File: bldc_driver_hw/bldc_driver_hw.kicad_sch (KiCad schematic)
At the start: 28 parts, among them J1 Conn_01x02, J10 MR60_F, J2 USB_C_Receptacle_USB2.0_16P, J3 JTAG_CONN, J4 USB_C_Receptacle_USB2.0_16P, J5 Conn_01x03_Pin, J6 Conn_01x03_Pin, J7 Conn_01x03, J9 Conn_01x02, U2 USBLC6-2SC6, U7 USBLC6-2SC6

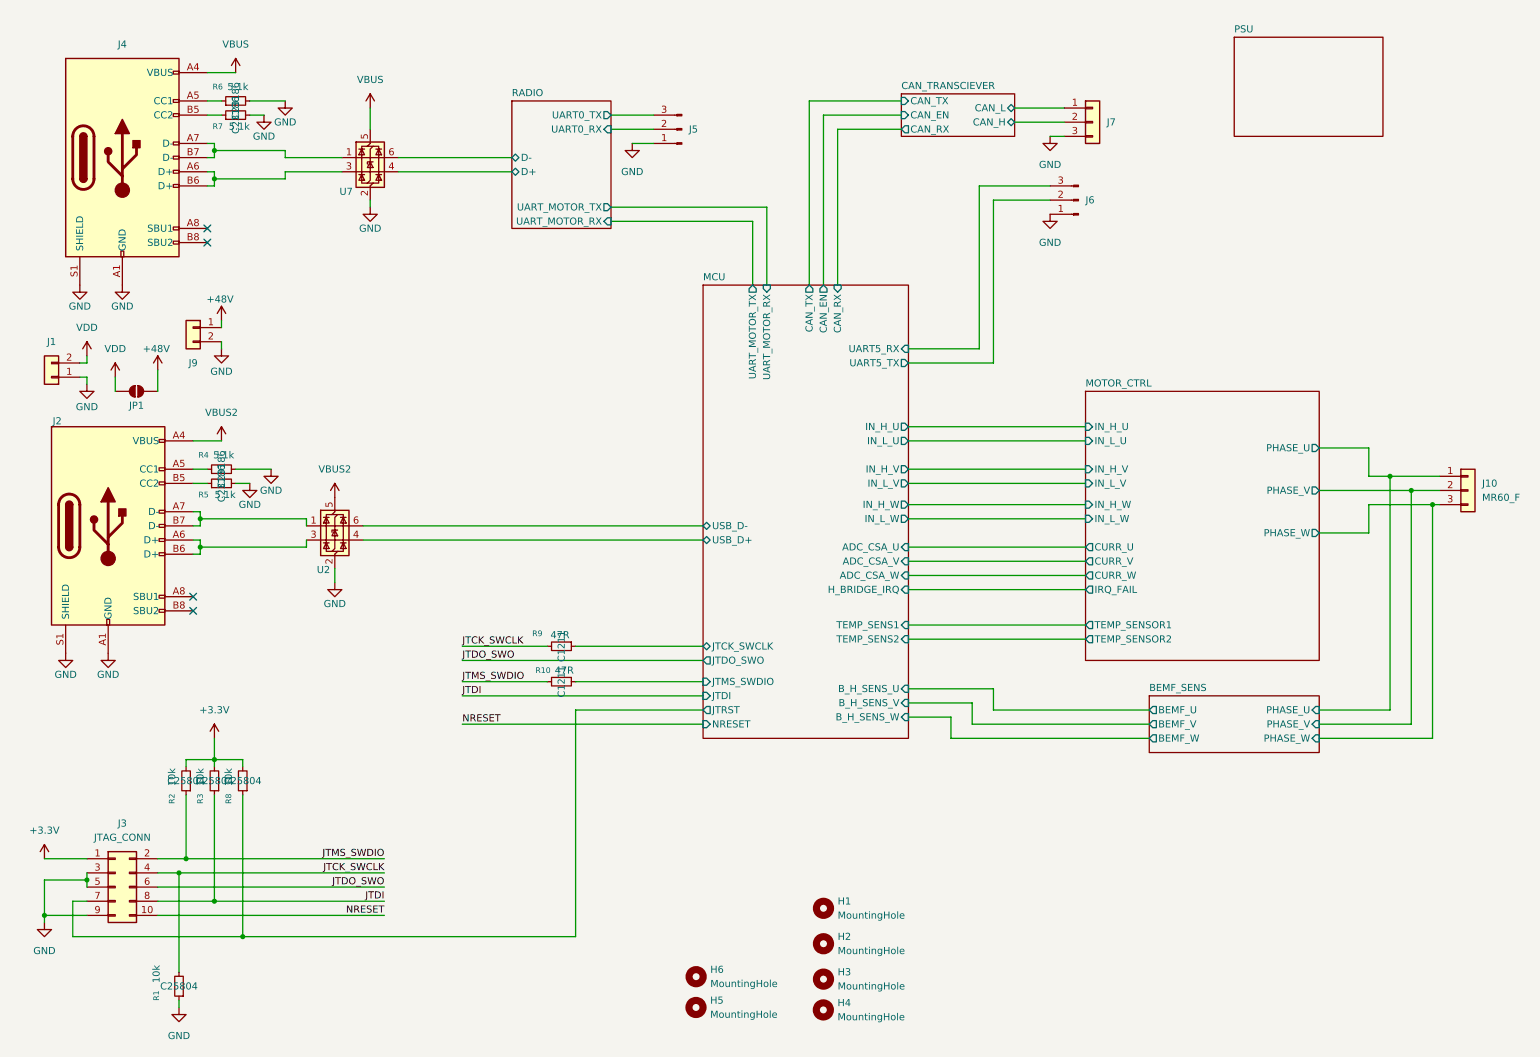
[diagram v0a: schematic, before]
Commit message: finished_board
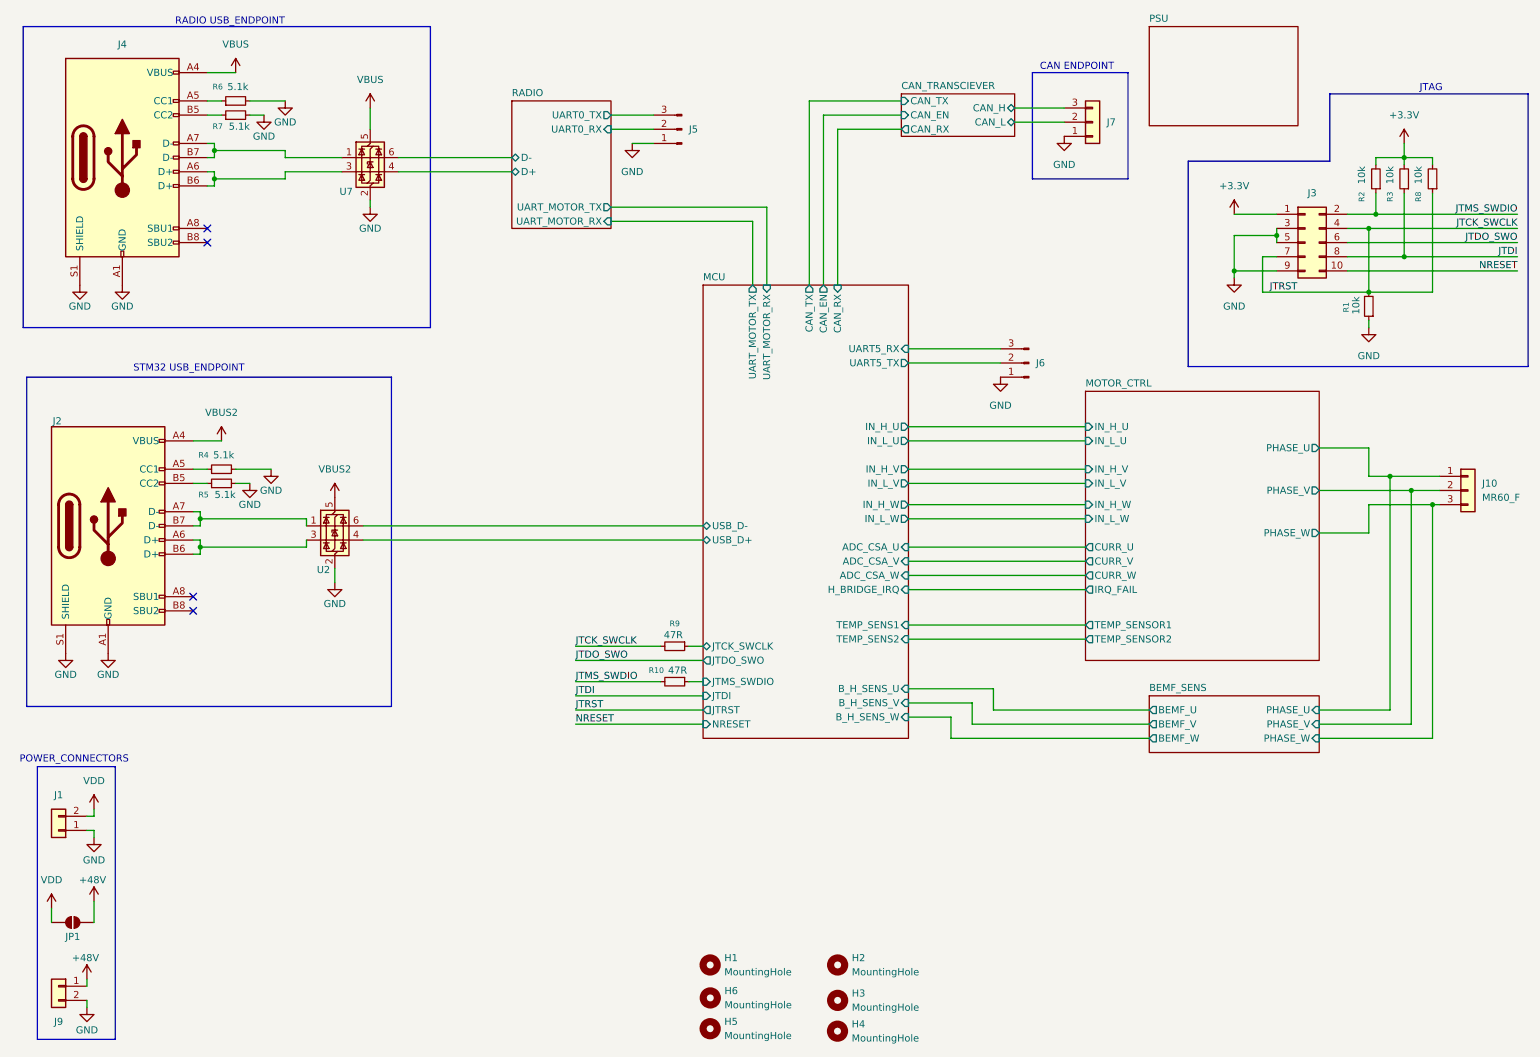
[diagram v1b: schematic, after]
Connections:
- net MCU/JTRST is gone; now on net JTCK_SWCLK: J3.7 (Pin_7), R8.1
- net CAN_TRANSCIEVER/CAN_H: now also J7.3 (Pin_3); no longer J7.2 (Pin_2)
- net CAN_TRANSCIEVER/CAN_L: now also J7.2 (Pin_2); no longer J7.1 (Pin_1)
- net GND: now also J7.1 (Pin_1); no longer J7.3 (Pin_3)
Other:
- note added: "CAN ENDPOINT"
- note added: "JTAG"
- note added: "POWER_CONNECTORS"
- note added: "RADIO USB_ENDPOINT"
- note added: "STM32 USB_ENDPOINT"
- moved on the sheet: H1, H2, H3, H4, H5, H6, J1, J3, J6, J9, JP1, R1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

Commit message: finished
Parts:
- J1, J10, J2, J3, J4, J5, J6, J7, J9, U2, U7: now left out of the parts list
- R10, R9: LCSC C1211 -> C23182
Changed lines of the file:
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@@
 		(unit 1)
 		(exclude_from_sim no)
-		(in_bom yes)
+		(in_bom no)
 		(on_board yes)
 		(dnp no)
@@
 			)
 		)
-		(property "LCSC" "C1211"
+		(property "LCSC" "C23182"
 			(at 130.81 132.08 0)
 			(effects
@@
 		(unit 1)
 		(exclude_from_sim no)
-		(in_bom yes)
+		(in_bom no)
 		(on_board yes)
 		(dnp no)
@@
 		(unit 1)
 		(exclude_from_sim no)
-		(in_bom yes)
+		(in_bom no)
 		(on_board yes)
 		(dnp no)
@@
 		(unit 1)
 		(exclude_from_sim no)
-		(in_bom yes)
+		(in_bom no)
 		(on_board yes)
 		(dnp no)
@@
 		(unit 1)
 		(exclude_from_sim no)
-		(in_bom yes)
+		(in_bom no)
 		(on_board yes)
 		(dnp no)
@@
 		(unit 1)
 		(exclude_from_sim no)
-		(in_bom yes)
+		(in_bom no)
 		(on_board yes)
 		(dnp no)
@@
 		(unit 1)
 		(exclude_from_sim no)
-		(in_bom yes)
+		(in_bom no)
 		(on_board yes)
 		(dnp no)
@@
 		(unit 1)
 		(exclude_from_sim no)
-		(in_bom yes)
+		(in_bom no)
 		(on_board yes)
 		(dnp no)
@@
 		(unit 1)
 		(exclude_from_sim no)
-		(in_bom yes)
+		(in_bom no)
 		(on_board yes)
 		(dnp no)
@@
 		(unit 1)
 		(exclude_from_sim no)
-		(in_bom yes)
+		(in_bom no)
 		(on_board yes)
 		(dnp no)
@@
 			)
 		)
-		(property "LCSC" "C1211"
+		(property "LCSC" "C23182"
 			(at 130.81 125.73 0)
 			(effects
@@
 		(unit 1)
 		(exclude_from_sim no)
-		(in_bom yes)
+		(in_bom no)
 		(on_board yes)
 		(dnp no)
